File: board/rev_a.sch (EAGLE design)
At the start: 12 parts, among them IC1 STM32-M-48, IC2 LM2936DT-5.0, IC3 MCP6004, Q1 35A/25V/8.5mΩ, U1 3.3V/150mA

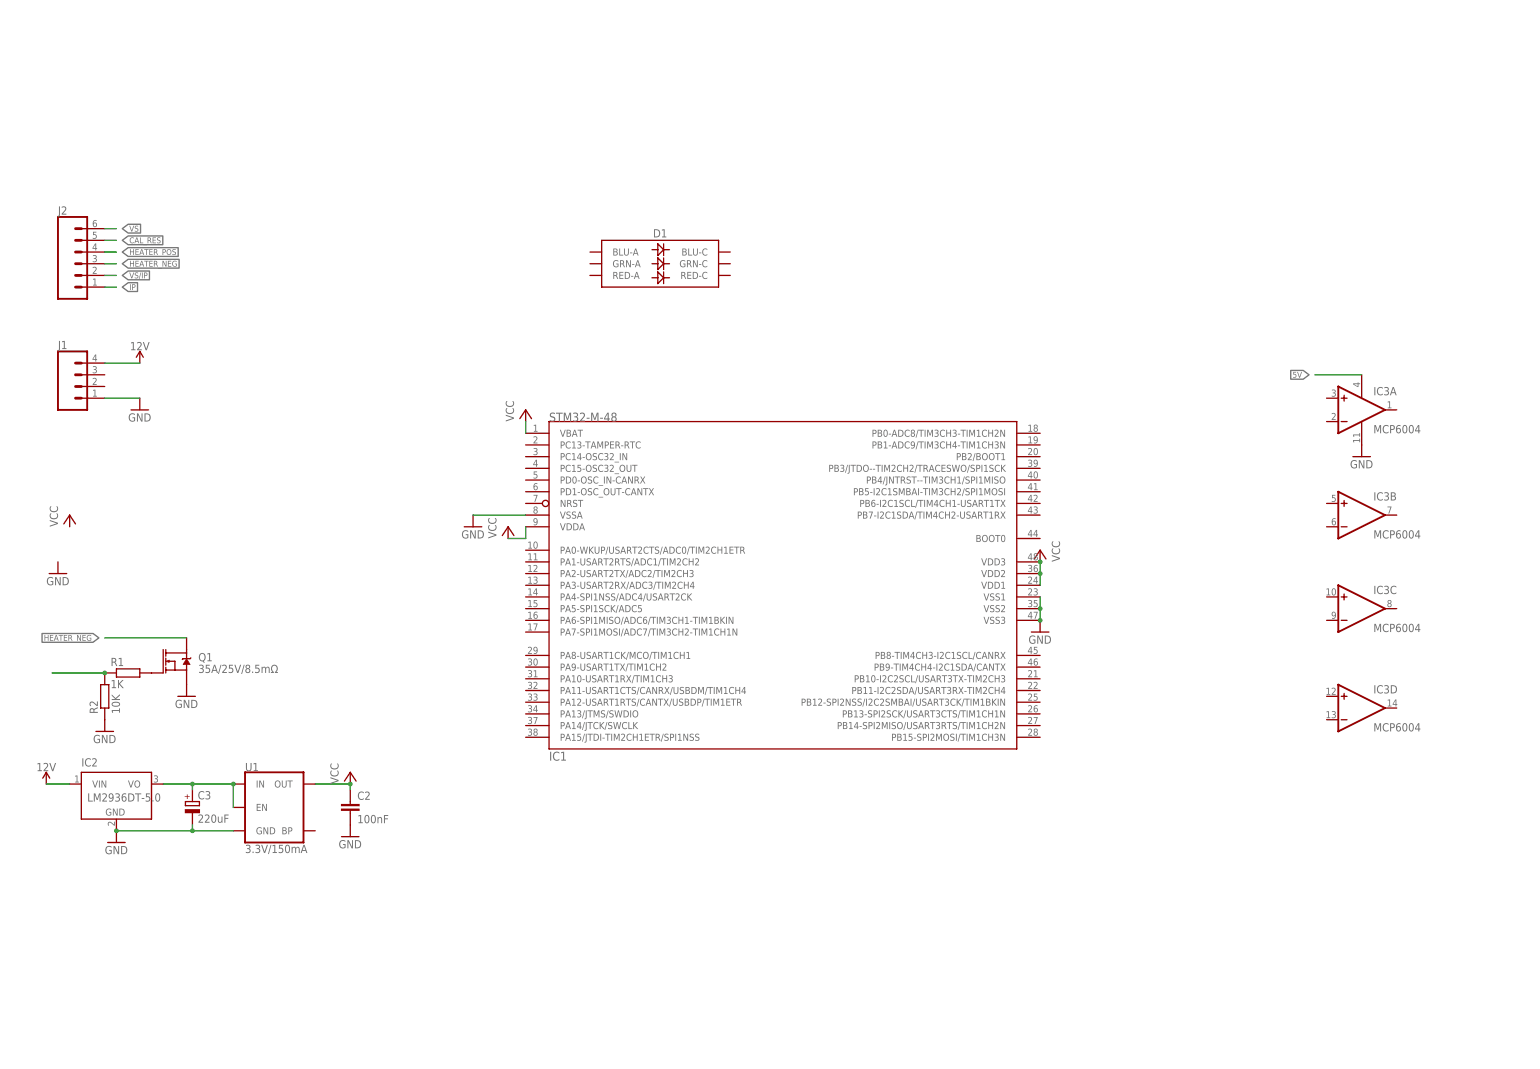
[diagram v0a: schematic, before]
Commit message: [board] Updated PCB and IOC files
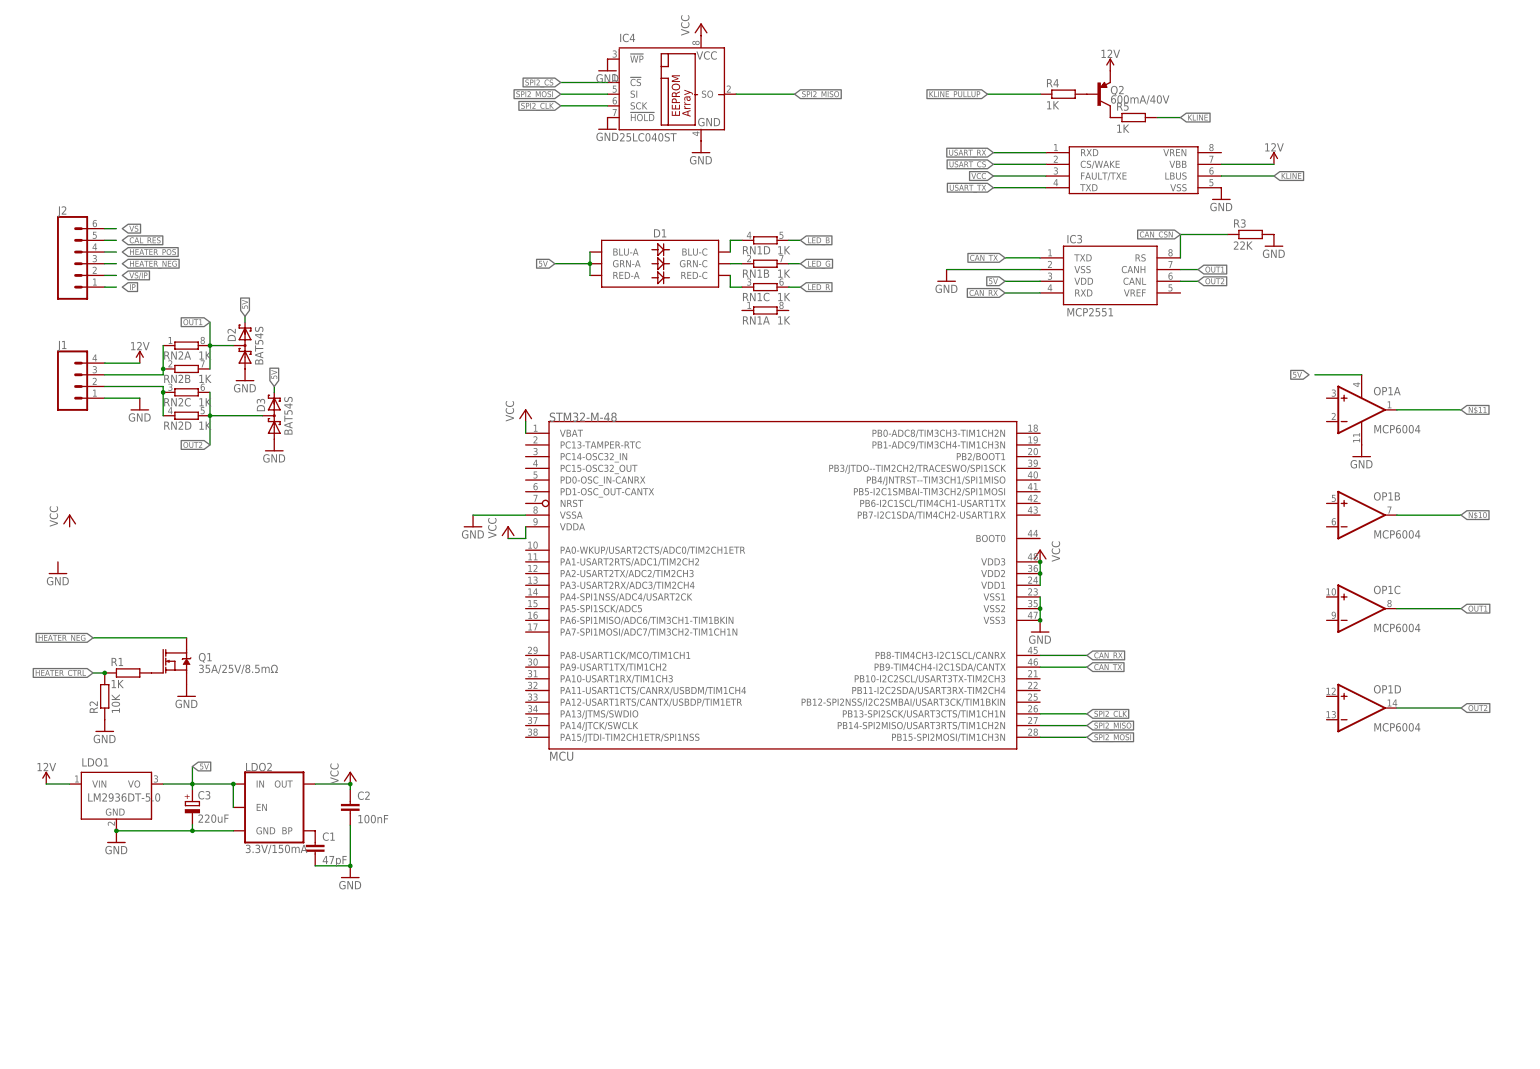
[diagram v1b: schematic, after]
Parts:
- added C1: 47pF, resistor:C-EUC0603
- added D2, D3: BAT54S, diode:BAT54S
- added IC4: 25LC040ST, microchip:25LC040ST
- added MCU: STM32-M-48, pel_stm32:STM32-M-48
- added OP1: MCP6004, linear:MCP604ST
- added Q2: 600mA/40V, SparkFun-DiscreteSemi:TRANS_PNP-MMBT4403
- added R3: 22K, resistor:R-EU_R0603
- added R4, R5: 1K, resistor:R-EU_R0603
- added RN1, RN2: 1K, resistor-dil:4R-N0603-ARC
- IC1: value STM32-M-48 -> TJA1027; device pel_stm32:STM32-M-48 -> misc:MCP2004
- IC3: value MCP6004 -> MCP2551; device linear:MCP604ST -> SparkFun-IC-Comms:MCP2551
- renumbered IC2 to LDO1, U1 to LDO2
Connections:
- net N$4 renamed HEATER_CTRL
- new net CAN_CSN: IC3.RS, R3.1
- new net CAN_RX: IC3.RXD, MCU.PB8-TIM4CH3-I2C1SCL/CANRX
- new net CAN_TX: IC3.TXD, MCU.PB9-TIM4CH4-I2C1SDA/CANTX
- new net KLINE: IC1.LBUS@6, R5.2
- new net KLINE_PULLUP: R4.1
- new net LED_B: RN1D.2
- new net LED_G: RN1B.2
- new net LED_R: RN1C.2
- new net N$1: Q2.C, R5.1
- new net N$10: OP1B.OUT
- new net N$11: OP1A.OUT
- new net N$3: D1.BLU-C, RN1D.1
- new net N$4: C1.1, LDO2.BP
- new net N$5: D1.GRN-C, RN1B.1
- new net N$6: D1.RED-C, RN1C.1
- new net N$7: Q2.B, R4.2
- new net OUT1: D2.C1A2, IC3.CANH, OP1C.OUT, RN2A.2, RN2B.2
- new net OUT1_C: J1.3, RN2A.1, RN2B.1
- new net OUT2: D3.C1A2, IC3.CANL, OP1D.OUT, RN2C.2, RN2D.2
- new net OUT2_C: J1.2, RN2C.1, RN2D.1
- new net SPI2_CLK: IC4.SCK, MCU.PB13-SPI2SCK/USART3CTS/TIM1CH1N
- new net SPI2_CS: IC4.!CS
- new net SPI2_MISO: IC4.SO, MCU.PB14-SPI2MISO/USART3RTS/TIM1CH2N
- new net SPI2_MOSI: IC4.SI, MCU.PB15-SPI2MOSI/TIM1CH3N
- new net USART_CS: IC1.CS/WAKE@2
- new net USART_RX: IC1.RXD@1
- new net USART_TX: IC1.TXD@4
- net 12V: now also IC1.VBB@7, Q2.E
- net 5V: now also D1.BLU-A, D1.RED-A, D2.C2, D3.C2, IC3.VDD, OP1P.V+; no longer IC3P.V+
- net GND: now also C1.2, D2.A1, D3.A1, IC1.VSS@5, IC3.VSS, IC4.!HOLD, IC4.!WP, IC4.GND, MCU.VSS1, MCU.VSS2, MCU.VSS3, OP1P.V-, R3.2; no longer IC1.VSS1, IC1.VSS2, IC1.VSS3, IC3P.V-
- net VBAT: now also MCU.VBAT; no longer IC1.VBAT
- net VCC: now also IC1.FAULT/TXE@3, IC4.VCC, MCU.VDD1, MCU.VDD2, MCU.VDD3, MCU.VDDA; no longer IC1.VDD1, IC1.VDD2, IC1.VDD3, IC1.VDDA
- net VSSA: now also MCU.VSSA; no longer IC1.VSSA

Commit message: [board] Cleaning up
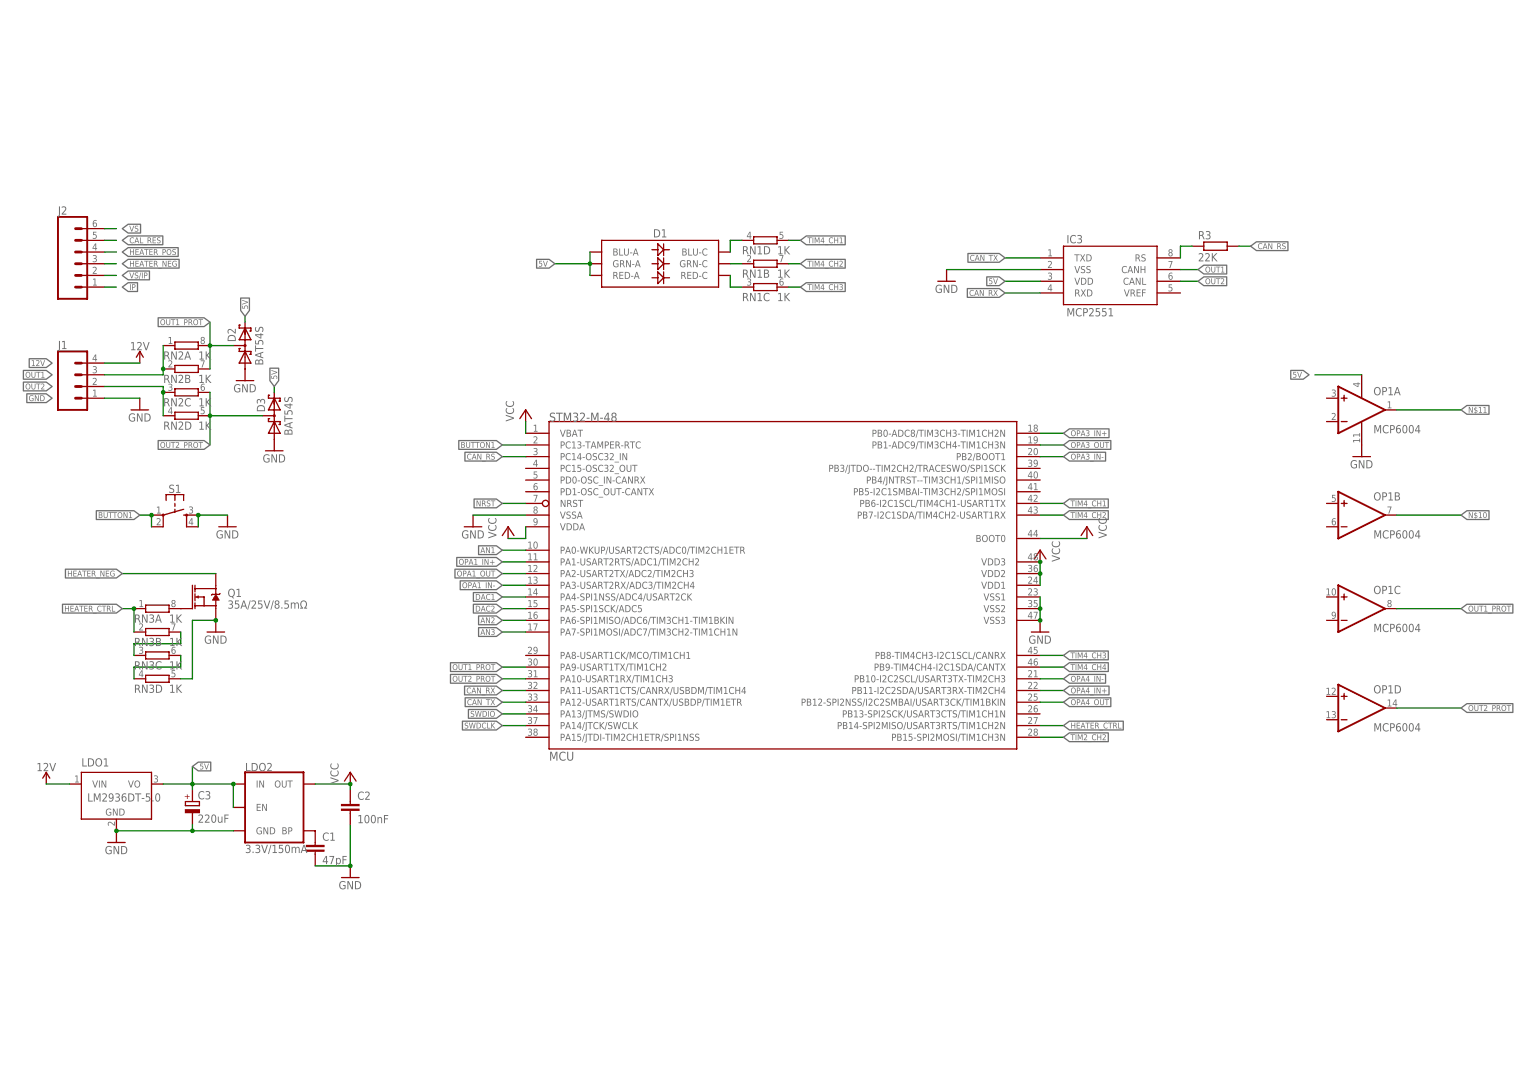
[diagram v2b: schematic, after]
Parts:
- removed IC1: TJA1027, misc:MCP2004
- removed IC4: 25LC040ST, microchip:25LC040ST
- removed Q2: 600mA/40V, SparkFun-DiscreteSemi:TRANS_PNP-MMBT4403
- removed R1, R4, R5: 1K, resistor:R-EU_R0603
- removed R2: 10K, resistor:R-EU_R0603
- added RN3: 1K, resistor-dil:4R-N0603-ARC
- added S1: (no value), SparkFun-Switches:MOMENTARY-SWITCH-SPST-2-SMD-5.2MM
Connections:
- net CAN_CSN renamed N$8
- removed net KLINE: IC1.LBUS@6, R5.2
- removed net KLINE_PULLUP: R4.1
- removed net LED_B: RN1D.2
- removed net LED_G: RN1B.2
- removed net LED_R: RN1C.2
- removed net OUT1_C: J1.3, RN2A.1, RN2B.1
- removed net OUT2_C: J1.2, RN2C.1, RN2D.1
- removed net SPI2_CLK: IC4.SCK, MCU.PB13-SPI2SCK/USART3CTS/TIM1CH1N
- removed net SPI2_CS: IC4.!CS
- removed net SPI2_MISO: IC4.SO, MCU.PB14-SPI2MISO/USART3RTS/TIM1CH2N
- removed net SPI2_MOSI: IC4.SI, MCU.PB15-SPI2MOSI/TIM1CH3N
- removed net USART_CS: IC1.CS/WAKE@2
- removed net USART_RX: IC1.RXD@1
- removed net USART_TX: IC1.TXD@4
- new net AN1: MCU.PA0-WKUP/USART2CTS/ADC0/TIM2CH1ETR
- new net AN2: MCU.PA6-SPI1MISO/ADC6/TIM3CH1-TIM1BKIN
- new net AN3: MCU.PA7-SPI1MOSI/ADC7/TIM3CH2-TIM1CH1N
- new net BUTTON1: MCU.PC13-TAMPER-RTC, S1.1, S1.2
- new net CAN_RS: MCU.PC14-OSC32_IN, R3.2
- new net DAC1: MCU.PA4-SPI1NSS/ADC4/USART2CK
- new net DAC2: MCU.PA5-SPI1SCK/ADC5
- new net NRST: MCU.NRST
- new net OPA1_IN+: MCU.PA1-USART2RTS/ADC1/TIM2CH2
- new net OPA1_IN-: MCU.PA3-USART2RX/ADC3/TIM2CH4
- new net OPA1_OUT: MCU.PA2-USART2TX/ADC2/TIM2CH3
- new net OPA3_IN+: MCU.PB0-ADC8/TIM3CH3-TIM1CH2N
- new net OPA3_IN-: MCU.PB2/BOOT1
- new net OPA3_OUT: MCU.PB1-ADC9/TIM3CH4-TIM1CH3N
- new net OPA4_IN+: MCU.PB11-I2C2SDA/USART3RX-TIM2CH4
- new net OPA4_IN-: MCU.PB10-I2C2SCL/USART3TX-TIM2CH3
- new net OPA4_OUT: MCU.PB12-SPI2NSS/I2C2SMBAI/USART3CK/TIM1BKIN
- new net OUT1_PROT: D2.C1A2, MCU.PA9-USART1TX/TIM1CH2, OP1C.OUT, RN2A.2, RN2B.2
- new net OUT2_PROT: D3.C1A2, MCU.PA10-USART1RX/TIM1CH3, OP1D.OUT, RN2C.2, RN2D.2
- new net SWDCLK: MCU.PA14/JTCK/SWCLK
- new net SWDIO: MCU.PA13/JTMS/SWDIO
- new net TIM2_CH2: MCU.PB15-SPI2MOSI/TIM1CH3N
- new net TIM4_CH1: MCU.PB6-I2C1SCL/TIM4CH1-USART1TX, RN1D.2
- new net TIM4_CH2: MCU.PB7-I2C1SDA/TIM4CH2-USART1RX, RN1B.2
- new net TIM4_CH3: MCU.PB8-TIM4CH3-I2C1SCL/CANRX, RN1C.2
- new net TIM4_CH4: MCU.PB9-TIM4CH4-I2C1SDA/CANTX
- net 12V: no longer IC1.VBB@7, Q2.E
- net 5V: now also D1.GRN-A
- net CAN_RX: now also MCU.PA11-USART1CTS/CANRX/USBDM/TIM1CH4; no longer MCU.PB8-TIM4CH3-I2C1SCL/CANRX
- net CAN_TX: now also MCU.PA12-USART1RTS/CANTX/USBDP/TIM1ETR; no longer MCU.PB9-TIM4CH4-I2C1SDA/CANTX
- net GND: now also RN3D.2, S1.3, S1.4; no longer IC1.VSS@5, IC4.!HOLD, IC4.!WP, IC4.GND, R2.1, R3.2
- net HEATER_CTRL: now also MCU.PB14-SPI2MISO/USART3RTS/TIM1CH2N, RN3A.1, RN3B.1; no longer R1.1, R2.2
- net N$1: now also Q1.G, RN3A.2; no longer Q2.C, R5.1
- net N$2: now also RN3B.2, RN3C.1; no longer Q1.G, R1.2
- net N$7: now also RN3C.2, RN3D.1; no longer Q2.B, R4.2
- net OUT1: now also J1.3, RN2A.1, RN2B.1; no longer D2.C1A2, OP1C.OUT, RN2A.2, RN2B.2
- net OUT2: now also J1.2, RN2C.1, RN2D.1; no longer D3.C1A2, OP1D.OUT, RN2C.2, RN2D.2
- net VCC: now also MCU.BOOT0; no longer IC1.FAULT/TXE@3, IC4.VCC
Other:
- moved on the sheet: Q1, R3

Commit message: [board] Testing a few configurations
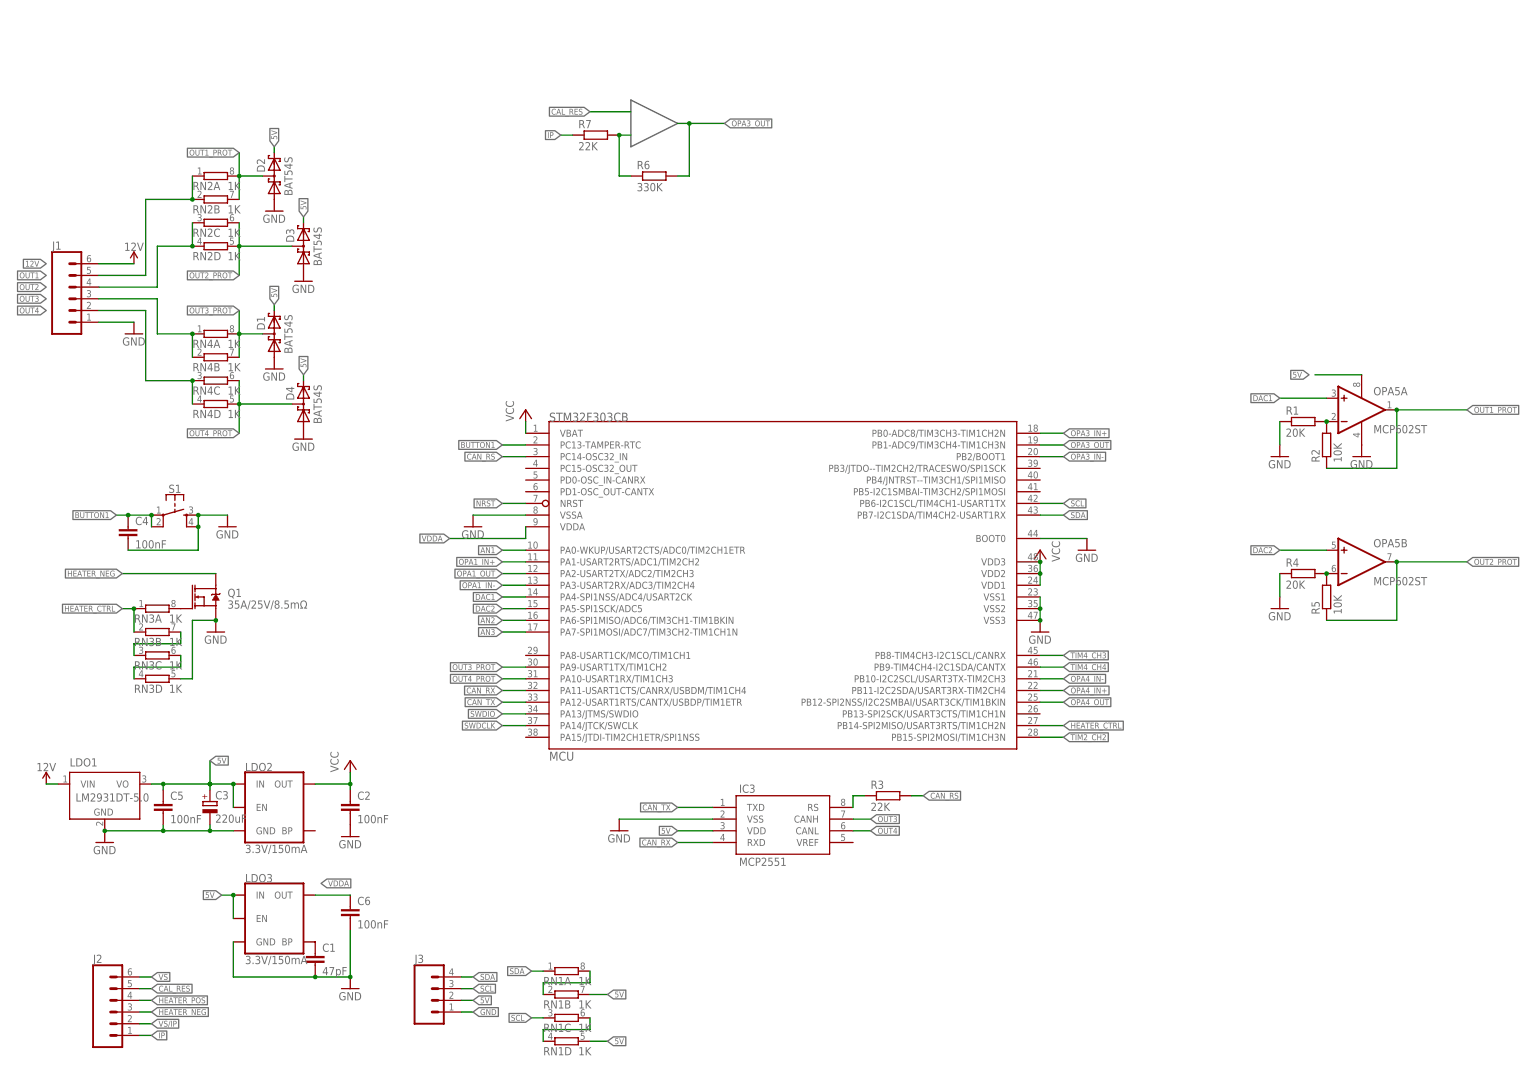
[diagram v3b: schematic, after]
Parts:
- removed OP1: MCP6004, linear:MCP604ST
- added C4, C5, C6: 100nF, resistor:C-EUC0603
- added D4: BAT54S, diode:BAT54S
- added J3: (no value), SparkFun-Connectors:CONN_04LOCK
- added LDO3: 3.3V/150mA, SparkFun-IC-Power:V_REG_MIC52053.3V
- added OPA5: MCP602ST, linear:MCP602ST
- added R1, R4: 20K, resistor:R-EU_R0603
- added R2, R5: 10K, resistor:R-EU_R0603
- added R6: 330K, resistor:R-EU_R0603
- added R7: 22K, resistor:R-EU_R0603
- added RN4: 1K, resistor-dil:4R-N0603-ARC
- D1: value (none) -> BAT54S; device SparkFun-LED:LED-RGBNO_IC -> diode:BAT54S
- J1: device SparkFun-Connectors:CONN_04LOCK_LONGPADS -> SparkFun-Connectors:CONN_06LONGPADS
- LDO1: value LM2936DT-5.0 -> LM2931DT-5.0
- MCU: value STM32-M-48 -> STM32F303CB
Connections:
- removed net N$4: C1.1, LDO2.BP
- removed net TIM4_CH1: MCU.PB6-I2C1SCL/TIM4CH1-USART1TX, RN1D.2
- removed net TIM4_CH2: MCU.PB7-I2C1SDA/TIM4CH2-USART1RX, RN1B.2
- new net N$9: RN1C.2, RN1D.1
- new net OUT3: IC3.CANH, J1.3, RN4A.1, RN4B.1
- new net OUT3_PROT: D1.C1A2, MCU.PA9-USART1TX/TIM1CH2, RN4A.2, RN4B.2
- new net OUT4: IC3.CANL, J1.2, RN4C.1, RN4D.1
- new net OUT4_PROT: D4.C1A2, MCU.PA10-USART1RX/TIM1CH3, RN4C.2, RN4D.2
- new net SCL: J3.3, MCU.PB6-I2C1SCL/TIM4CH1-USART1TX, RN1C.1
- new net SDA: J3.4, MCU.PB7-I2C1SDA/TIM4CH2-USART1RX, RN1A.1
- new net VDDA: C6.1, LDO3.OUT, MCU.VDDA
- net 12V: now also J1.6; no longer J1.4
- net 5V: now also C5.1, D1.C2, D4.C2, J3.2, LDO3.EN, LDO3.IN, OPA5P.V+, RN1B.2, RN1D.2; no longer D1.BLU-A, D1.GRN-A, D1.RED-A, OP1P.V+
- net BUTTON1: now also C4.1
- net DAC1: now also OPA5A.+IN
- net DAC2: now also OPA5B.+IN
- net GND: now also C4.2, C5.2, C6.2, D1.A1, D4.A1, J3.1, LDO3.GND, MCU.BOOT0, OPA5P.V-, R1.1, R4.1; no longer OP1P.V-
- net IP: now also R7.1
- net N$10: now also R6.1, R7.2; no longer OP1B.OUT
- net N$11: now also C1.1, LDO3.BP; no longer OP1A.OUT
- net N$3: now also RN1A.2, RN1B.1; no longer D1.BLU-C, RN1D.1
- net N$5: now also OPA5A.-IN, R1.2, R2.2; no longer D1.GRN-C, RN1B.1
- net N$6: now also R4.2, R5.2; no longer D1.RED-C, RN1C.1
- net OPA3_OUT: now also R6.2
- net OUT1: now also J1.5; no longer IC3.CANH, J1.3
- net OUT1_PROT: now also OPA5A.OUT, R2.1; no longer MCU.PA9-USART1TX/TIM1CH2, OP1C.OUT
- net OUT2: now also J1.4; no longer IC3.CANL, J1.2
- net OUT2_PROT: now also OPA5B.OUT, R5.1; no longer MCU.PA10-USART1RX/TIM1CH3, OP1D.OUT
- net TIM4_CH3: no longer RN1C.2
- net VCC: no longer MCU.BOOT0, MCU.VDDA
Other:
- note added: "OPA3"
- note added: "Pump cell current"
- moved on the sheet: C1, C3, D2, D3, IC3, J2, LDO1, R3, RN1B, RN1C, RN1D, RN2A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
